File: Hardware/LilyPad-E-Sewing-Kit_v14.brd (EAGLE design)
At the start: 51.1 x 52 mm, 47 parts

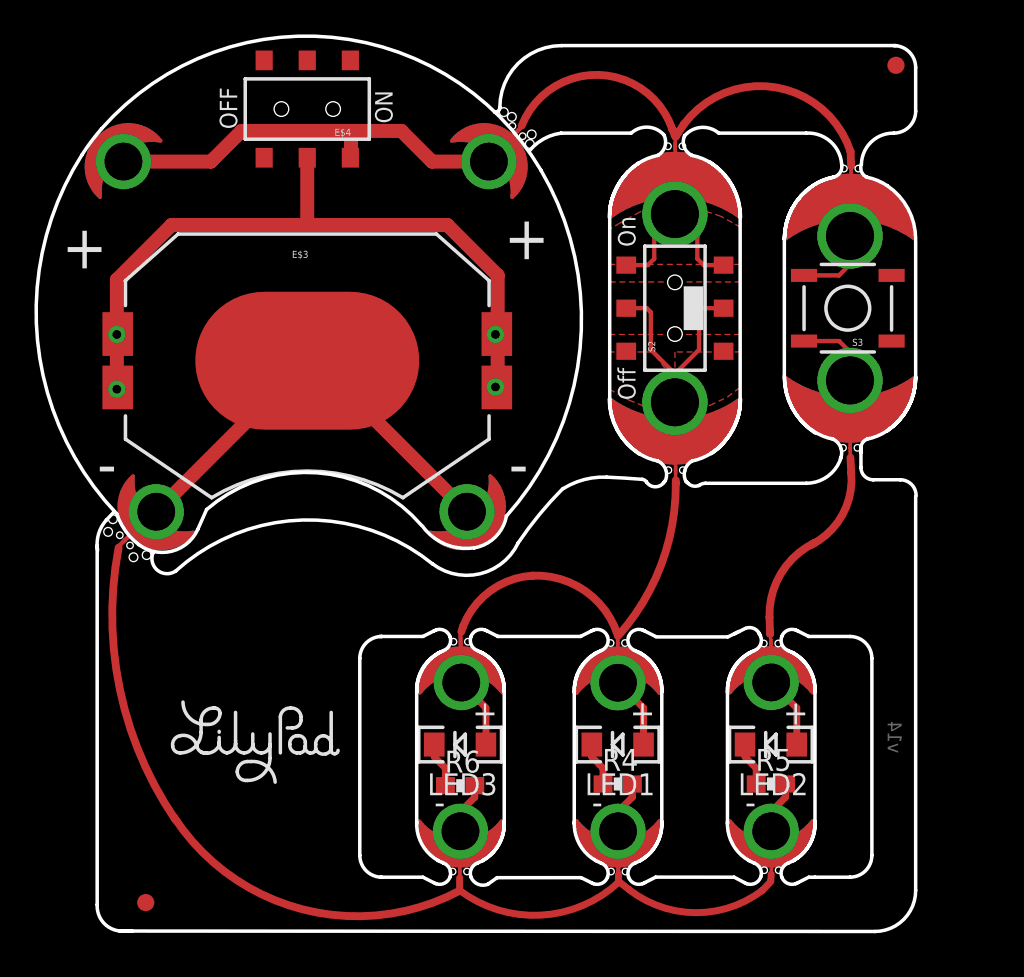
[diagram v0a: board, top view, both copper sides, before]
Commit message: Updated Brd and Sch files (in Sync)
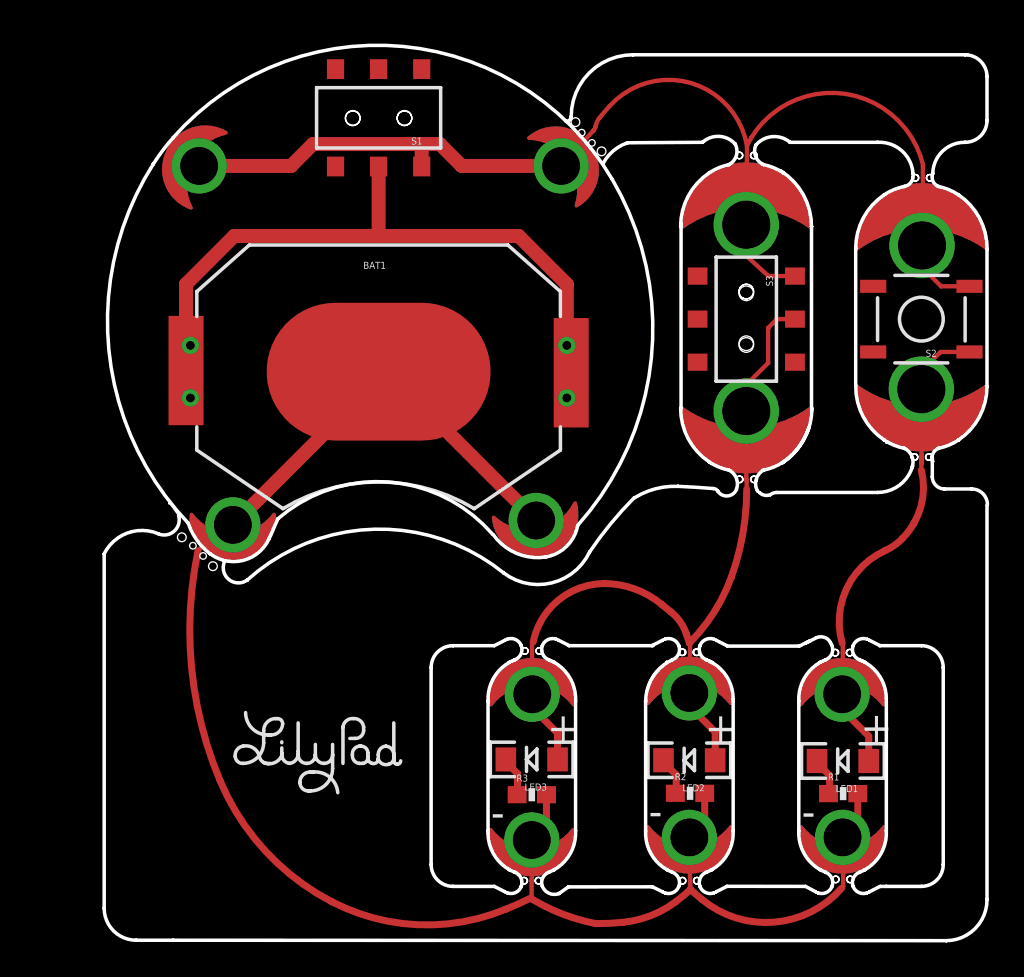
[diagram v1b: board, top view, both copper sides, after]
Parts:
- removed BUTTON-2, BUTTONS2, SLIDEOFF2, SLIDEON2: SEWTAP8, LilyPad-Wearables:PETAL-MEDIUM-2SIDE
- removed E$1: (no value), SparkFun-Aesthetics:CREATIVE_COMMONS
- removed E$2: (no value), SparkFun-Aesthetics:REVISION
- removed E$3: (no value), SparkFun-Electromechanical:BATTCON_20MM_4LEGS_OVERPASTE
- removed E$4: (no value), SparkFun-Electromechanical:AYZ0202
- removed E$5: (no value), LilyPad-Wearables:LOGO-LILYPAD
- removed JP1, JP2: FIDUCIAL1X2, SparkFun:FIDUCIAL-1X2
- removed LOGO1, LOGO2, LOGO3, LOGO4, LOGO5: LOGO-LPL, LilyPad-Wearables:LOGO-L
- removed R4, R5, R6: 150, SparkFun:0603-RES
- removed U$10, U$16, U$17, U$9: MOUSE-BITE-12_HOLES, Testing:MOUST-BITE-1-(2_HOLES)
- removed U$11, U$12, U$13, U$14: SEWTAP6, LilyPad-Wearables:PETAL-SMALL-2SIDE
- removed U$15: LOGO-LPLP, LilyPad-Wearables:LOGO-LILYPAD
- added BAT1: 20mm coincell, SparkFun-Electromechanical:BATTCON_20MM_4LEGS
- added BATB-, BATB-2, BATT+, BATT+2: SEWTAP6, LilyPad-Wearables:PETAL-SMALL-2SIDE
- added BUTTON-, BUTTONS, SLIDEOFF, SLIDEON: SEWTAP8, LilyPad-Wearables:PETAL-MEDIUM-2SIDE
- added FRAME1: FRAME-LETTER, SparkFun-Aesthetics:CREATIVE_COMMONS
- added MB+, MB-, MB1, MB10, MB2, MB3, MB4, MB5, MB6, MB7, MB8, MB9: MOUSE-BITE-12_HOLES, Testing:MOUST-BITE-1-(2_HOLES)
- added R1, R2, R3: 150, SparkFun-Resistors:0603-RES
- added S1: (no value), SparkFun-Electromechanical:AYZ0202
- LED1, LED2, LED3: value White -> WHITE; device SparkFun-3-2-07:LED-1206 -> SparkFun-LED:LED-1206
- S2: value AYZ0202 -> SWITCH-MOMENTARY-2SMD; device SparkFun:AYZ0202 -> SparkFun-Electromechanical:TACTILE-SWITCH-SMD
- S3: device SparkFun:TACTILE_SWITCH_SMD -> SparkFun-Electromechanical:AYZ0202
- U$1: value MOUSE-BITE-12_HOLES -> REVISION; device Testing:MOUST-BITE-1-(2_HOLES) -> SparkFun-Aesthetics:REVISION
- U$2, U$3: value MOUSE-BITE-12_HOLES -> (none); device Testing:MOUST-BITE-1-(2_HOLES) -> LilyPad-Wearables:LOGO-LILYPAD
- U$4, U$7, U$8: value MOUSE-BITE-12_HOLES -> (none); device Testing:MOUST-BITE-1-(2_HOLES) -> LilyPad-Wearables:LOGO-L-TINY
- U$5, U$6: value MOUSE-BITE-12_HOLES -> (none); device Testing:MOUST-BITE-1-(2_HOLES) -> LilyPad-Wearables:LOGO-L
- moved U$7 39.1 mm to (25.0, 9.94), turned to 0 degrees
- moved U$6 36.6 mm to (47.8, 35.5)
- moved U$1 35.9 mm to (0.14, -12.4), flipped to the top, turned to 0 degrees
- moved U$5 32.3 mm to (37.7, 35.9)
- moved U$2 26.9 mm to (12.8, 10.7), flipped to the top, turned to 0 degrees
- moved U$3 23.9 mm to (16.1, 36.1), turned to 0 degrees
- moved U$4 23.1 mm to (43.1, 9.96)
- moved U$8 20.4 mm to (34.2, 9.97)
- moved S2 14.3 mm to (47.8, 35.6), turned to 180 degrees
- moved LED1 13.1 mm to (43.2, 9.92)
- moved LED-1 13.0 mm to (43.2, 5.49)
- moved LED+1 13.0 mm to (43.2, 13.8)
- moved S3 5.93 mm to (37.6, 35.6), turned to 270 degrees
- moved LED2 4.82 mm to (34.3, 9.96)
- moved LED+2 4.79 mm to (34.3, 13.9)
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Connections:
- removed net BUTTON2: BUTTONS2.1, S3.2, U$8.P$1
- removed net GND2: U$11.1, U$13.1
- removed net N$4: LED1.C, R4.1
- removed net N$5: LED2.C, R5.1
- removed net N$6: LED3.C, R6.1
- removed net S$16: LED+2.1, LED2.A
- removed net S$2: U$14.1
- removed net S$25: U$2.P$1
- removed net S$26: LED+1.1, LED1.A, U$3.P$1
- removed net S$5: LED-3.1, R6.2, U$4.P$1
- removed net S$6: LED-1.1, R4.2
- removed net S$7: LED-2.1, R5.2, U$5.P$1
- removed net S$8: LED+3.1, LED3.A
- removed net SINK1: S2.4
- removed net SINK2: S2.1
- removed net SWITCH2: S2.2, S2.5, SLIDEOFF2.1, U$9.P$1
- removed net VCC2: BUTTON-2.1, S2.3, S2.6, S3.4, SLIDEON2.1, U$10.P$1, U$7.P$1
- new net BUTTON: BUTTONS.1, LED+1.1, LED1.A, MB3.P$1, MB9.P$1, S2.1
- new net GND: BAT1.NEGATIVE, BATB-.1, BATB-2.1, LED-1.1, LED-2.1, LED-3.1, MB-.P$1, MB6.P$1, MB7.P$1, MB8.P$1, R1.2, R2.2, R3.2
- new net N$1: BAT1.POSITIVE@1, BAT1.POSITIVE@2, BAT1.POSITIVE@3, BAT1.POSITIVE@4, S1.2
- new net N$11: LED1.C, R1.1
- new net N$12: LED2.C, R2.1
- new net N$13: LED3.C, R3.1
- new net N$2: BATT+.1, BATT+2.1, BUTTON-.1, MB+.P$1, MB1.P$1, S1.1, S2.3, S3.1, SLIDEON.1
- new net SWITCH: LED+2.1, LED+3.1, LED2.A, LED3.A, MB10.P$1, MB4.P$1, MB5.P$1, S3.2, SLIDEOFF.1
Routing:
- net GND: track 0.00 -> 100.4 mm
- net N$2: track 0.00 -> 65.7 mm
- net SWITCH: track 0.00 -> 48.0 mm
- net N$1: track 0.00 -> 44.2 mm, vias 0 -> 4
- net VCC2: track 34.4 -> 0.00 mm
- net BUTTON: track 0.00 -> 28.3 mm
- net S$2: track 25.6 -> 0.00 mm
- net GND2: track 25.2 -> 0.00 mm
- net S$4: track 23.1 -> 0.00 mm
- net S$10: track 19.9 -> 0.00 mm, vias 2 -> 0
- net S$29: track 19.2 -> 0.00 mm
- net SWITCH2: track 17.7 -> 0.00 mm
- net S$18: track 17.1 -> 0.00 mm
- net S$28: track 16.1 -> 0.00 mm
- net S$23: track 11.3 -> 0.00 mm
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- removed copper zone on layer 1, net GND2
- removed copper zone on layer 1, net SINK1
- removed copper zone on layer 1, net SINK2
- removed copper zone on layer 1, net VCC2
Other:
- board size 51.1 x 52 mm -> 51.4 x 52 mm
- board text added: "All Units Inches"
- board text added: "Board Thickness: "0.032""
- board text added: "M. West"
- board text removed: "All Units inches"
- board text removed: "Board Thickness: 0.032""
- board text removed: "Mary West"
- board text removed: "OFF"
- board text removed: "ON"
- board text removed: "Off"
- board text removed: "On"
- board text removed: "White"
- board text removed: "v14"
